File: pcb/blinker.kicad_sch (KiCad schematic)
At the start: 14 parts, among them J1 ISP, U1 ATtiny10-TS

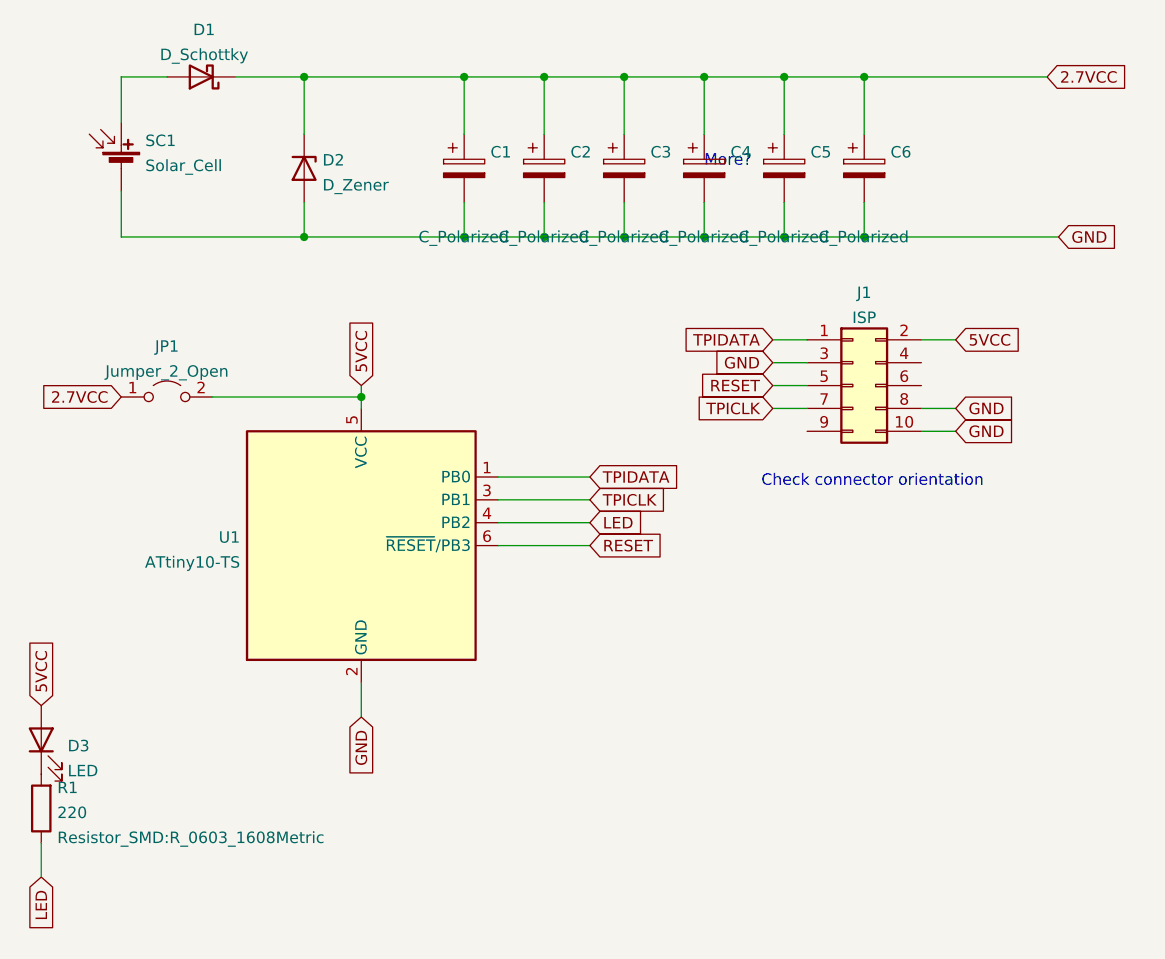
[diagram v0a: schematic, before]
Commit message: About to route PCB.
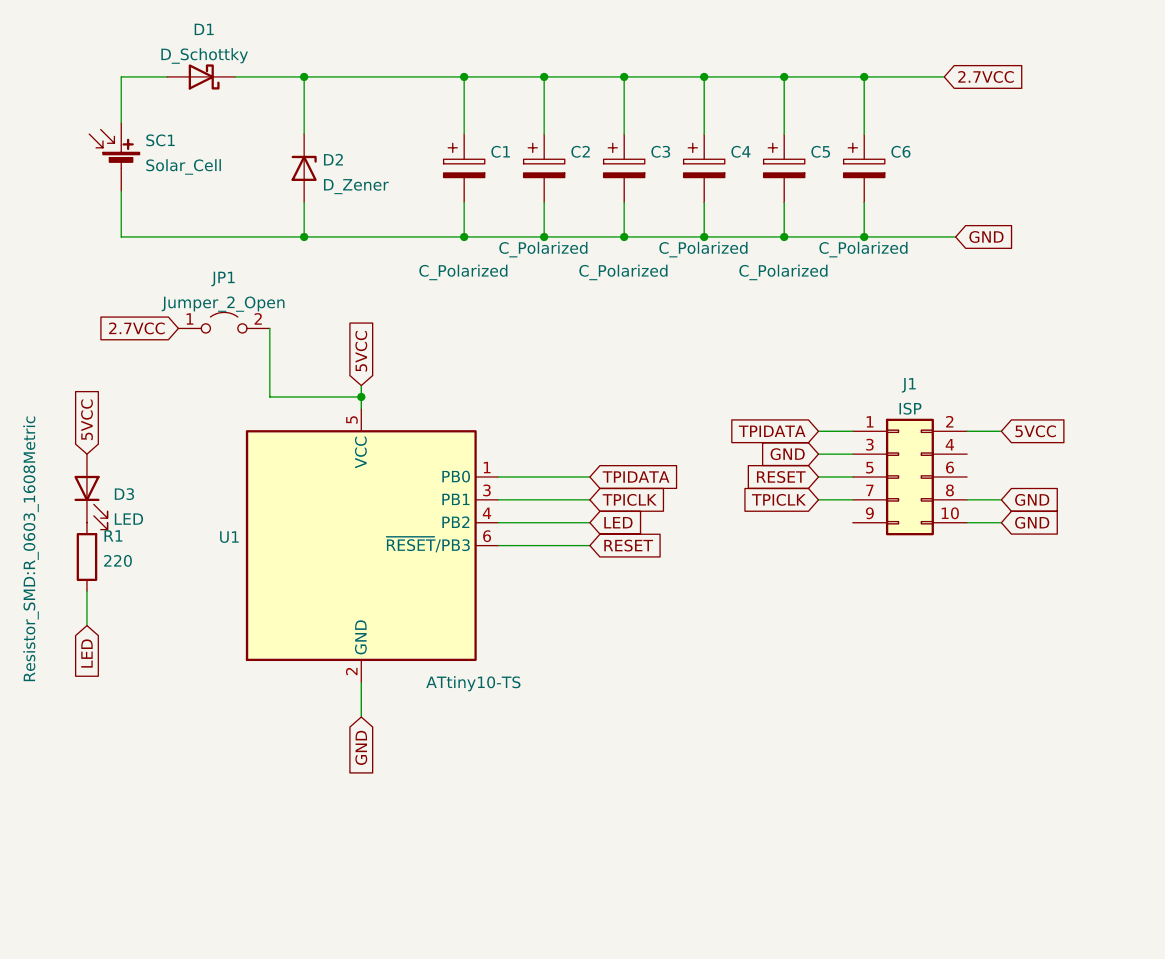
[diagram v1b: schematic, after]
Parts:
- D2: footprint Diode_SMD:D_SOD-123 -> Diode_SMD:D_SOD-123F; LCSC C707156 -> C362294
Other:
- note removed: "Check connector orientation"
- note removed: "More?"
- moved on the sheet: D3, J1, JP1, R1

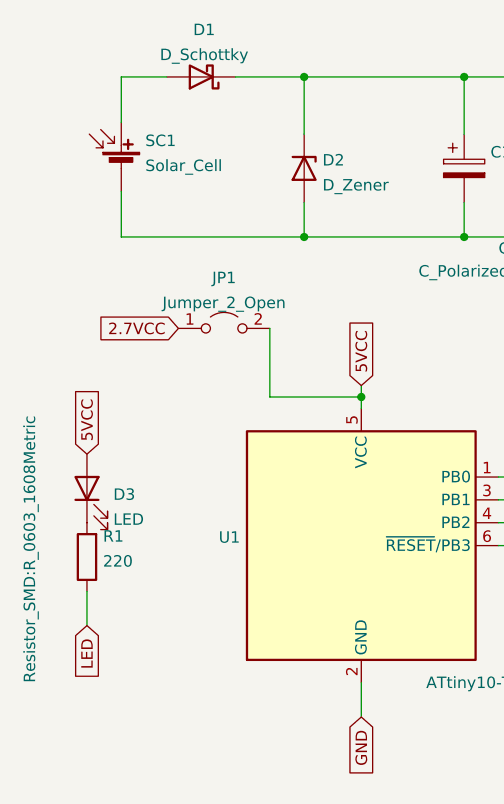
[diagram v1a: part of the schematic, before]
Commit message: Routed
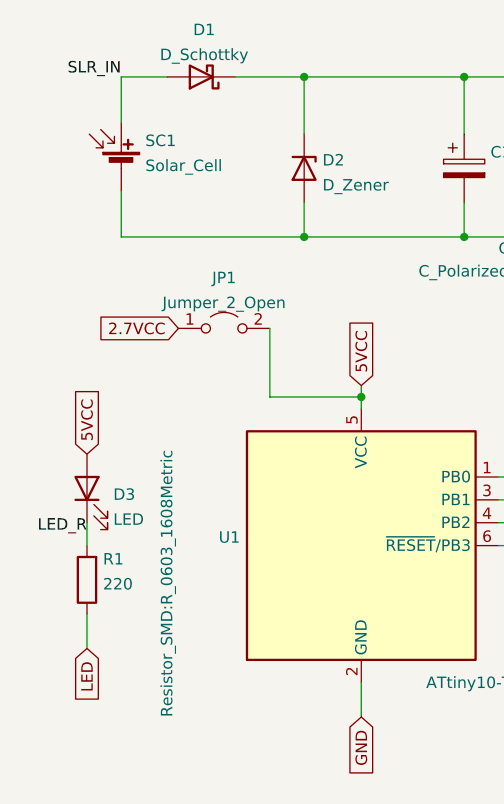
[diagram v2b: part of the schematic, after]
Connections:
- net LED_R: now reaches D3.1 (K), R1.2
- net SLR_IN: now reaches D1.2 (A), SC1.1 (+)
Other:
- moved on the sheet: R1
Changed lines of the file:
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@@
     (stroke (width 0) (type default) (color 0 0 0 0))
   )
-  (wire (pts (xy 59.69 119.38) (xy 59.69 123.19))
+  (wire (pts (xy 59.69 121.92) (xy 59.69 125.73))
     (stroke (width 0) (type default) (color 0 0 0 0))
   )
@@
     (stroke (width 0) (type default) (color 0 0 0 0))
   )
+  (wire (pts (xy 59.69 114.3) (xy 59.69 111.76))
+    (stroke (width 0) (type default) (color 0 0 0 0))
+  )
   (wire (pts (xy 137.16 80.01) (xy 146.05 80.01))
     (stroke (width 0) (type default) (color 0 0 0 0))
@@
   (wire (pts (xy 101.6 62.23) (xy 110.49 62.23))
     (stroke (width 0) (type default) (color 0 0 0 0))
+  )
+  (label "LED_R" (at 59.69 113.03 180)
+    (effects (font (size 1.27 1.27)) (justify right bottom))
+  )
+  (label "SLR_IN" (at 63.5 62.23 180)
+    (effects (font (size 1.27 1.27)) (justify right bottom))
   )
   (global_label "TPICLK" (shape input) (at 140.97 109.22 180) (fields_autoplaced)
@@
     )
   )
-  (global_label "LED" (shape input) (at 59.69 123.19 270) (fields_autoplaced)
+  (global_label "LED" (shape input) (at 59.69 125.73 270) (fields_autoplaced)
     (effects (font (size 1.27 1.27)) (justify right))
-    (property "Intersheet References" "${INTERSHEET_REFS}" (id 0) (at 59.7694 129.0502 90)
+    (property "Intersheet References" "${INTERSHEET_REFS}" (id 0) (at 59.7694 131.5902 90)
       (effects (font (size 1.27 1.27)) (justify right) hide)
     )
   )
-  (symbol (lib_id "Device:R") (at 59.69 115.57 180) (unit 1)
+  (symbol (lib_id "Device:R") (at 59.69 118.11 180) (unit 1)
     (in_bom yes) (on_board yes)
-    (property "Reference" "R1" (id 0) (at 61.468 113.2739 0)
+    (property "Reference" "R1" (id 0) (at 61.468 115.8139 0)
       (effects (font (size 1.27 1.27)) (justify right))
     )
-    (property "Value" "220" (id 1) (at 61.468 116.049 0)
+    (property "Value" "220" (id 1) (at 61.468 118.589 0)
       (effects (font (size 1.27 1.27)) (justify right))
     )
-    (property "Footprint" "Resistor_SMD:R_0603_1608Metric" (id 2) (at 53.34 129.54 90)
+    (property "Footprint" "Resistor_SMD:R_0603_1608Metric" (id 2) (at 68.58 133.35 90)
       (effects (font (size 1.27 1.27)) (justify right))
     )
-    (property "Datasheet" "~" (id 3) (at 59.69 115.57 0)
+    (property "Datasheet" "~" (id 3) (at 59.69 118.11 0)
       (effects (font (size 1.27 1.27)) hide)
     )
-    (property "JLC" "C22962" (id 4) (at 59.69 115.57 0)
+    (property "JLC" "C22962" (id 4) (at 59.69 118.11 0)
       (effects (font (size 1.27 1.27)) hide)
     )
